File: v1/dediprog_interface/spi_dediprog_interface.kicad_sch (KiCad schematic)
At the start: 3 parts, among them J1 Conn_02x10_Odd_Even, J2 Conn_01x02_Pin, J4 Conn_01x10_Socket

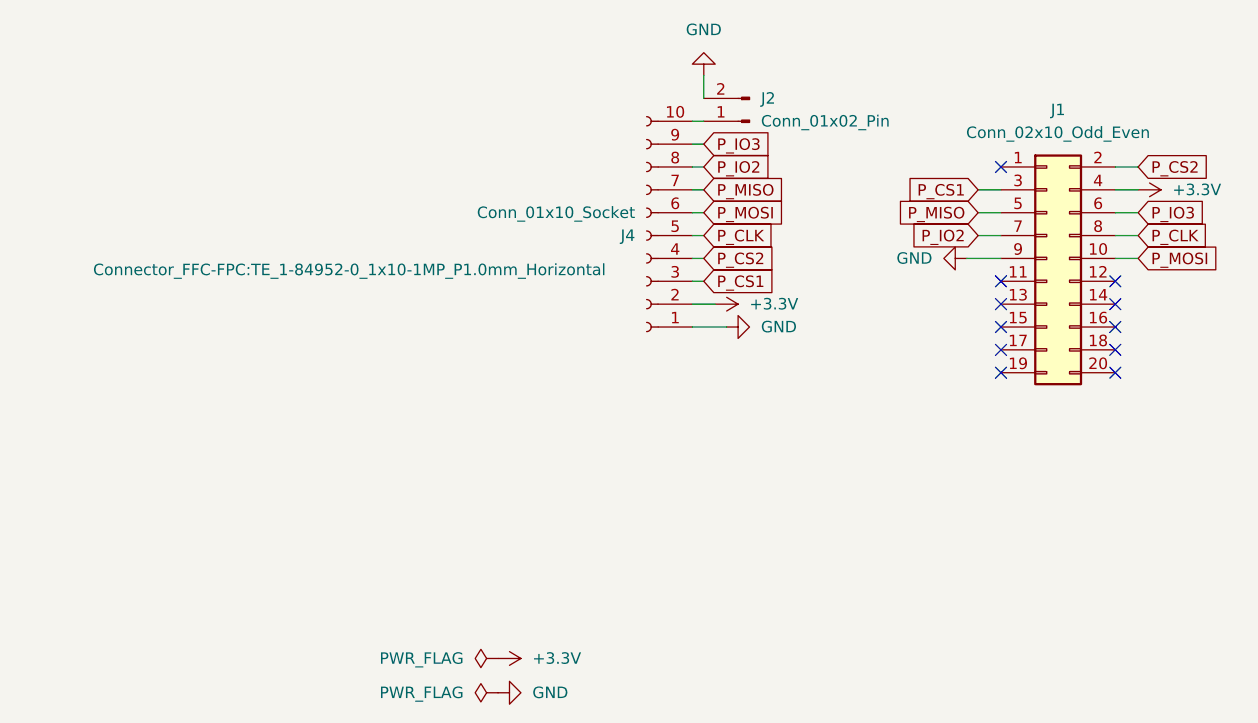
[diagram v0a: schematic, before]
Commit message: WIP: Redesign
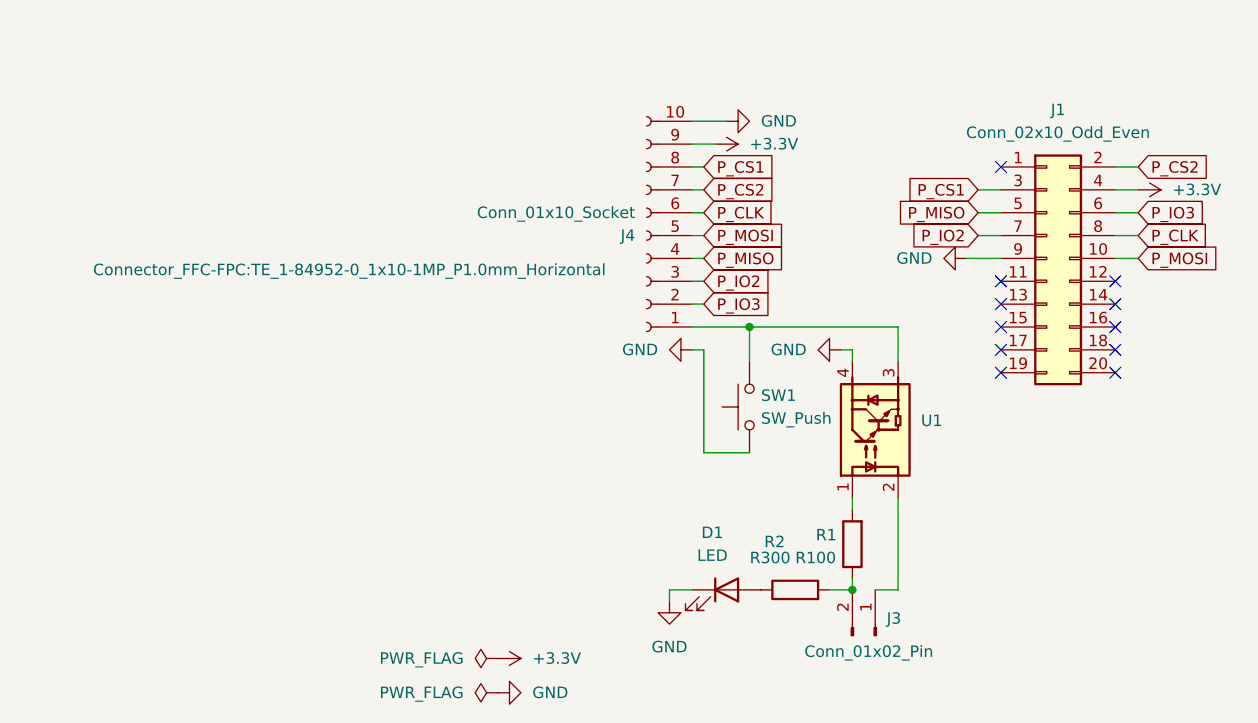
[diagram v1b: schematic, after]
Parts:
- removed J2: Conn_01x02_Pin, Connector_PinHeader_2.54mm:PinHeader_1x02_P2.54mm_Vertical, symbol Connector:Conn_01x02_Pin
- added D1: LED, LED_SMD:LED_0805_2012Metric, symbol Device:LED
- added J3: Conn_01x02_Pin, Connector_PinHeader_2.54mm:PinHeader_1x02_P2.54mm_Vertical, symbol Connector:Conn_01x02_Pin
- added R1: R100, Resistor_SMD:R_0805_2012Metric, symbol Device:R
- added R2: R300, Resistor_SMD:R_0805_2012Metric, symbol Device:R
- added SW1: SW_Push, Button_Switch_SMD:SW_Tactile_SPST_NO_Straight_CK_PTS636Sx25SMTRLFS, symbol Switch:SW_Push
- added U1: ~, Package_DIP:SMDIP-4_W7.62mm, symbol custom:TLP3556A
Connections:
- net +3.3V: now also J4.9 (Pin_9); no longer J4.2 (Pin_2)
- net GND: now also J4.10 (Pin_10), D1.1 (K), SW1.1, U1.4; no longer J4.1 (Pin_1)
- net P_CLK: now also J4.6 (Pin_6); no longer J4.5 (Pin_5)
- net P_CS1: now also J4.8 (Pin_8); no longer J4.3 (Pin_3)
- net P_CS2: now also J4.7 (Pin_7); no longer J4.4 (Pin_4)
- net P_IO2: now also J4.3 (Pin_3); no longer J4.8 (Pin_8)
- net P_IO3: now also J4.2 (Pin_2); no longer J4.9 (Pin_9)
- net P_MISO: now also J4.4 (Pin_4); no longer J4.7 (Pin_7)
- net P_MOSI: now also J4.5 (Pin_5); no longer J4.6 (Pin_6)
- new net: J3.1 (Pin_1), U1.2
- new net: J3.2 (Pin_2), R1.1, R2.2
- new net: R1.2, U1.1
- new net: J4.1 (Pin_1), SW1.2, U1.3
- new net: D1.2 (A), R2.1
